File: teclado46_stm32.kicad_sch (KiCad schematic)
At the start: 11 parts, among them U1 XC6206PxxxMR, U2 STM32G474CETx, U4 W25Q128JVS

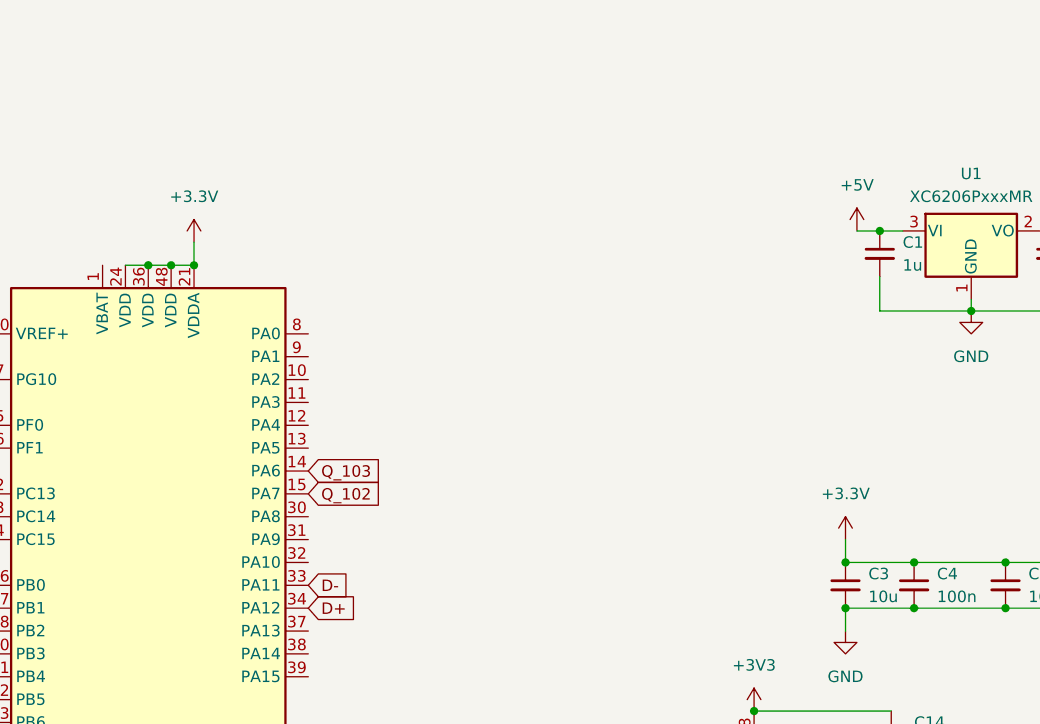
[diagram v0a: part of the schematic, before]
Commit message: chore: routed caps, flash and regulator
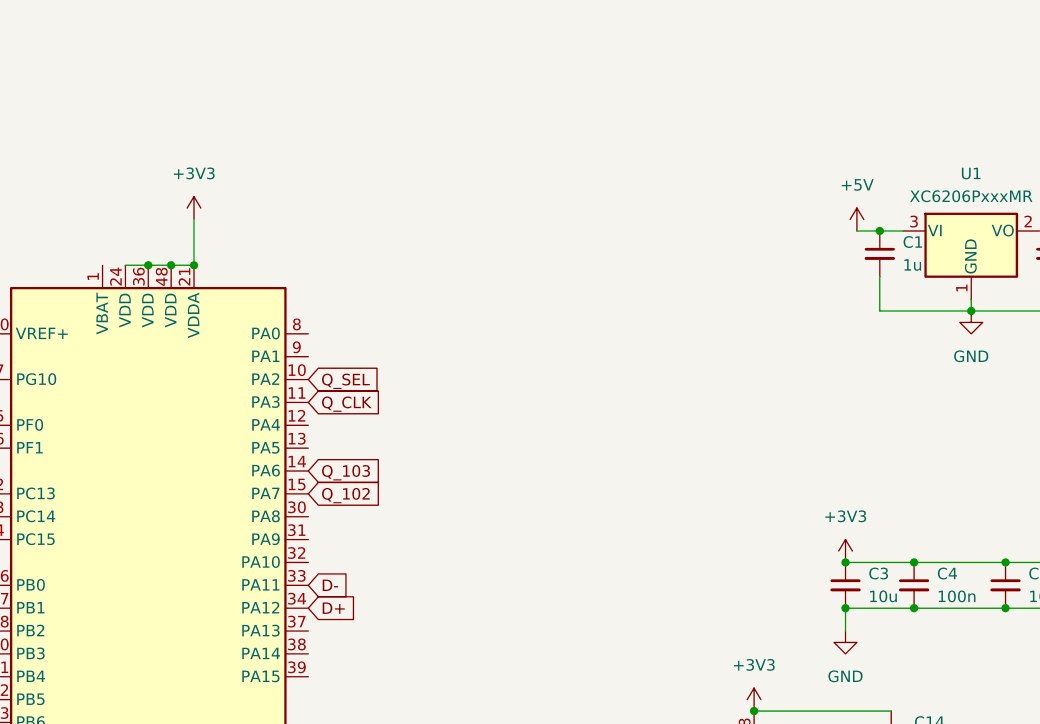
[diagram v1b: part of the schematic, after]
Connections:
- net +3.3V is gone; now on net +3V3: C3.1, C4.1, C5.1, C6.1, C7.1, U2.21 (VDDA), U2.24 (VDD), U2.36 (VDD), U2.48 (VDD)
- net Q_CLK: now also U2.11 (PA3)
- net Q_SEL: now also U2.10 (PA2)
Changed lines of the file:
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@@
+	)
+	(junction
+		(at 55.88 102.87)
+		(diameter 0)
+		(color 0 0 0 0)
 	)
 	(junction
@@
 	)
 	(junction
-		(at 55.88 102.87)
-		(diameter 0)
-		(color 0 0 0 0)
-	)
-	(junction
 		(at 156.21 140.97)
 		(diameter 0)
@@
 	(wire
 		(pts
-			(xy 55.88 100.33) (xy 55.88 102.87)
-		)
-		(stroke
-			(width 0)
-			(type default)
-		)
-	)
-	(wire
-		(pts
 			(xy 128.27 143.51) (xy 128.27 140.97)
 		)
@@
 	(wire
 		(pts
+			(xy 55.88 97.79) (xy 55.88 102.87)
+		)
+		(stroke
+			(width 0)
+			(type default)
+		)
+	)
+	(wire
+		(pts
 			(xy 128.27 140.97) (xy 135.89 140.97)
 		)
@@
 	(wire
 		(pts
-			(xy 128.27 133.35) (xy 128.27 135.89)
-		)
-		(stroke
-			(width 0)
-			(type default)
-		)
-	)
-	(wire
-		(pts
 			(xy 132.08 104.14) (xy 132.08 107.95)
 		)
@@
 			(width 0)
 			(type default)
+		)
+	)
+	(global_label "Q_SEL"
+		(shape input)
+		(at 68.58 115.57 0)
+		(fields_autoplaced yes)
+		(effects
+			(font
+				(size 1.27 1.27)
+			)
+			(justify left)
+		)
+		(property "Intersheetrefs" "${INTERSHEET_REFS}"
+			(at 77.2499 115.57 0)
+			(effects
+				(font
+					(size 1.27 1.27)
+				)
+				(justify left)
+				(hide yes)
+			)
 		)
 	)
@@
 				)
 				(justify right)
+				(hide yes)
+			)
+		)
+	)
+	(global_label "Q_CLK"
+		(shape input)
+		(at 68.58 118.11 0)
+		(fields_autoplaced yes)
+		(effects
+			(font
+				(size 1.27 1.27)
+			)
+			(justify left)
+		)
+		(property "Intersheetrefs" "${INTERSHEET_REFS}"
+			(at 77.4314 118.11 0)
+			(effects
+				(font
+					(size 1.27 1.27)
+				)
+				(justify left)
 				(hide yes)
 			)
@@
 	)
 	(symbol
+		(lib_id "power:+3V3")
+		(at 128.27 135.89 0)
+		(unit 1)
+		(exclude_from_sim no)
+		(in_bom yes)
+		(on_board yes)
+		(dnp no)
+		(fields_autoplaced yes)
+		(property "Reference" "#PWR05"
+			(at 128.27 139.7 0)
+			(effects
+				(font
+					(size 1.27 1.27)
+				)
+				(hide yes)
+			)
+		)
+		(property "Value" "+3V3"
+			(at 128.27 130.81 0)
+			(effects
+				(font
+					(size 1.27 1.27)
+				)
+			)
+		)
+		(property "Footprint" ""
+			(at 128.27 135.89 0)
+			(effects
+				(font
+					(size 1.27 1.27)
+				)
+				(hide yes)
+			)
+		)
+		(property "Datasheet" ""
+			(at 128.27 135.89 0)
+			(effects
+				(font
+					(size 1.27 1.27)
+				)
+				(hide yes)
+			)
+		)
+		(property "Description" "Power symbol creates a global label with name \"+3V3\""
+			(at 128.27 135.89 0)
+			(effects
+				(font
+					(size 1.27 1.27)
+				)
+				(hide yes)
+			)
+		)
+		(pin "1"
+		)
+		(instances
+			(project "teclado46_stm32"
+				(path "/6ed4739c-92e8-425a-abb0-74006c04cb3a"
+					(reference "#PWR05")
+					(unit 1)
+				)
+			)
+		)
+	)
+	(symbol
 		(lib_id "power:GND")
 		(at 128.27 143.51 0)
@@
 	)
 	(symbol
-		(lib_id "power:+3.3V")
-		(at 55.88 100.33 0)
-		(unit 1)
-		(exclude_from_sim no)
-		(in_bom yes)
-		(on_board yes)
-		(dnp no)
-		(fields_autoplaced yes)
-		(property "Reference" "#PWR03"
-			(at 55.88 104.14 0)
-			(effects
-				(font
-					(size 1.27 1.27)
-				)
-				(hide yes)
-			)
-		)
-		(property "Value" "+3.3V"
-			(at 55.88 95.25 0)
-			(effects
-				(font
-					(size 1.27 1.27)
-				)
-			)
-		)
-		(property "Footprint" ""
-			(at 55.88 100.33 0)
-			(effects
-				(font
-					(size 1.27 1.27)
-				)
-				(hide yes)
-			)
-		)
-		(property "Datasheet" ""
-			(at 55.88 100.33 0)
-			(effects
-				(font
-					(size 1.27 1.27)
-				)
-				(hide yes)
-			)
-		)
-		(property "Description" "Power symbol creates a global label with name \"+3.3V\""
-			(at 55.88 100.33 0)
-			(effects
-				(font
-					(size 1.27 1.27)
-				)
-				(hide yes)
-			)
-		)
-		(pin "1"
-		)
-		(instances
-			(project ""
-				(path "/6ed4739c-92e8-425a-abb0-74006c04cb3a"
-					(reference "#PWR03")
-					(unit 1)
-				)
-			)
-		)
-	)
-	(symbol
 		(lib_id "power:+5V")
 		(at 129.54 99.06 0)
@@
 	)
 	(symbol
-		(lib_id "power:+3.3V")
-		(at 128.27 133.35 0)
+		(lib_id "power:+3V3")
+		(at 55.88 97.79 0)
 		(unit 1)
 		(exclude_from_sim no)
@@
 		(dnp no)
 		(fields_autoplaced yes)
-		(property "Reference" "#PWR05"
-			(at 128.27 137.16 0)
-			(effects
-				(font
-					(size 1.27 1.27)
-				)
-				(hide yes)
-			)
-		)
-		(property "Value" "+3.3V"
-			(at 128.27 128.27 0)
+		(property "Reference" "#PWR03"
+			(at 55.88 101.6 0)
+			(effects
+				(font
+					(size 1.27 1.27)
+				)
+				(hide yes)
+			)
+		)
+		(property "Value" "+3V3"
+			(at 55.88 92.71 0)
 			(effects
 				(font
@@
 		)
 		(property "Footprint" ""
-			(at 128.27 133.35 0)
+			(at 55.88 97.79 0)
 			(effects
 				(font
@@
 		)
 		(property "Datasheet" ""
-			(at 128.27 133.35 0)
-			(effects
-				(font
-					(size 1.27 1.27)
-				)
-				(hide yes)
-			)
-		)
-		(property "Description" "Power symbol creates a global label with name \"+3.3V\""
-			(at 128.27 133.35 0)
+			(at 55.88 97.79 0)
+			(effects
+				(font
+					(size 1.27 1.27)
+				)
+				(hide yes)
+			)
+		)
+		(property "Description" "Power symbol creates a global label with name \"+3V3\""
+			(at 55.88 97.79 0)
 			(effects
 				(font
@@
 			(project "teclado46_stm32"
 				(path "/6ed4739c-92e8-425a-abb0-74006c04cb3a"
-					(reference "#PWR05")
+					(reference "#PWR03")
 					(unit 1)
 				)
